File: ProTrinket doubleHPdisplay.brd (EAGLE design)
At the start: 17.8 x 37.3 mm, 14 parts

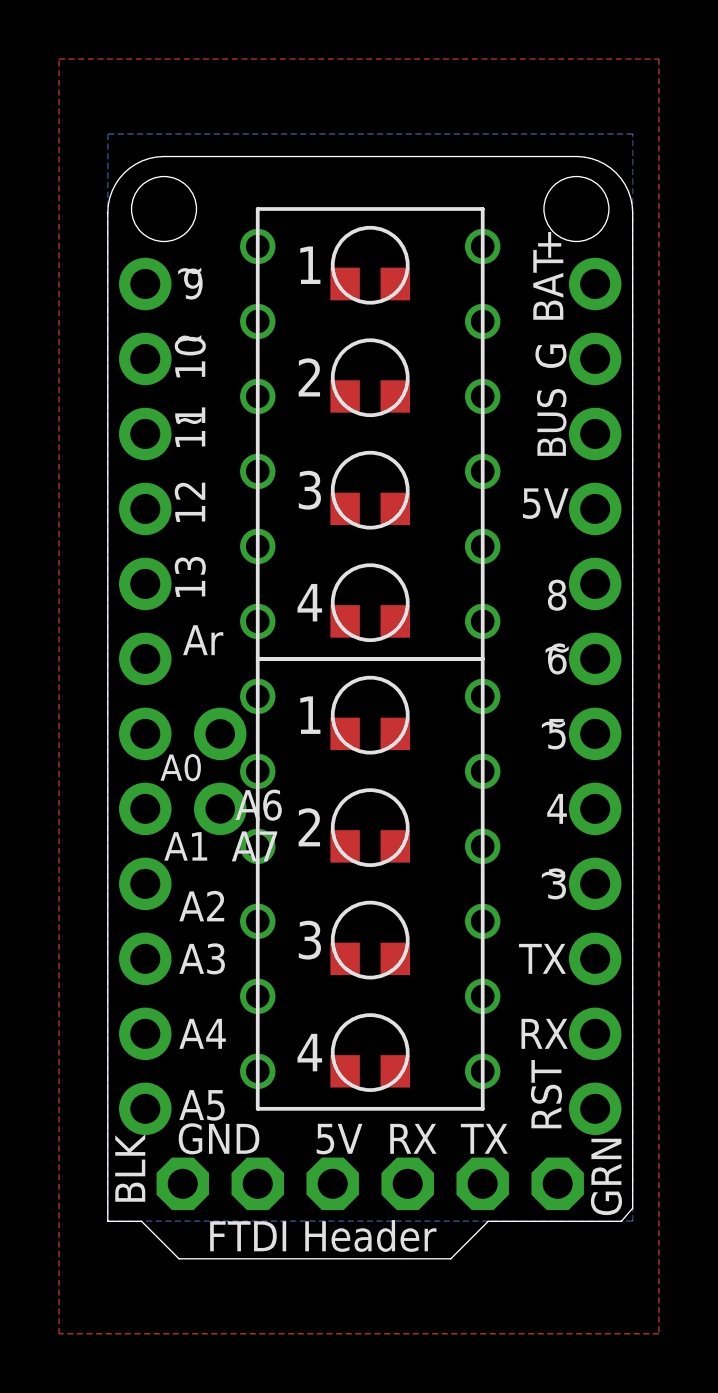
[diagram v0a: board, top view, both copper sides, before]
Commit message: routed board (thx jaromir)
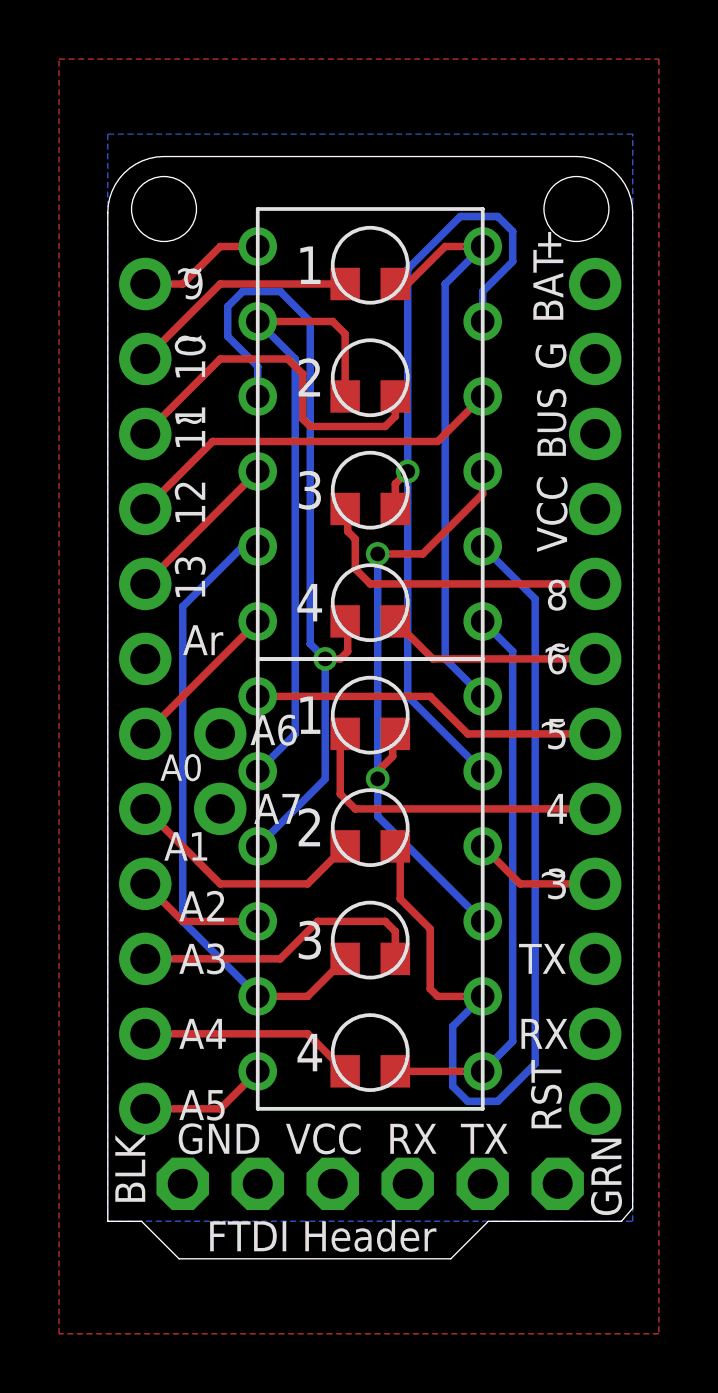
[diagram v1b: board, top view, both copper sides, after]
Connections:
- net A0: now also U$1.CAT_4
- net A1: now also R4.2
- net A2: now also U$2.CAT_3
- net A3: now also R8.2
- net A4: now also R7.2
- net A5: now also U$2.CAT_4
- net D10: now also R1.2
- net D11: now also R5.2
- net D12: now also U$1.CAT_2
- net D13: now also U$1.CAT_3
- net D3: now also U$2.CAT_2
- net D4: now also R6.2
- net D5: now also U$2.CAT_1
- net D6: now also R3.2
- net D8: now also R2.2
- net D9: now also U$1.CAT_1
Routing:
- net AD: track 0.00 -> 32.5 mm
- net AC: track 0.00 -> 27.8 mm, vias 0 -> 1
- net AB: track 0.00 -> 27.5 mm, vias 0 -> 1
- net AE: track 0.00 -> 21.5 mm
- net ADP: track 0.00 -> 21.1 mm
- net AF: track 0.00 -> 20.8 mm, vias 0 -> 2
- net AA: track 0.00 -> 19.8 mm
- net AG: track 0.00 -> 19.0 mm
- net D12: track 0.00 -> 13.0 mm
- net D11: track 0.00 -> 12.2 mm
- net D5: track 0.00 -> 12.0 mm
- net D4: track 0.00 -> 10.9 mm
- net D8: track 0.00 -> 10.5 mm
- net A3: track 0.00 -> 10.1 mm
- net A1: track 0.00 -> 8.35 mm
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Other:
- board text added: "VCC"
- board text added: "hackaday.io/davedarko"
- board text added: "special thanks for routing: hackaday.io/jaromir"
- board text removed: "5V"
- board text removed: "c"
